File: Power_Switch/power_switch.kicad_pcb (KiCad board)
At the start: 2 copper layers, 22 x 19.2 mm, 6 parts, among them J1 Conn_01x03_Pin, SW1 SW_SPDT

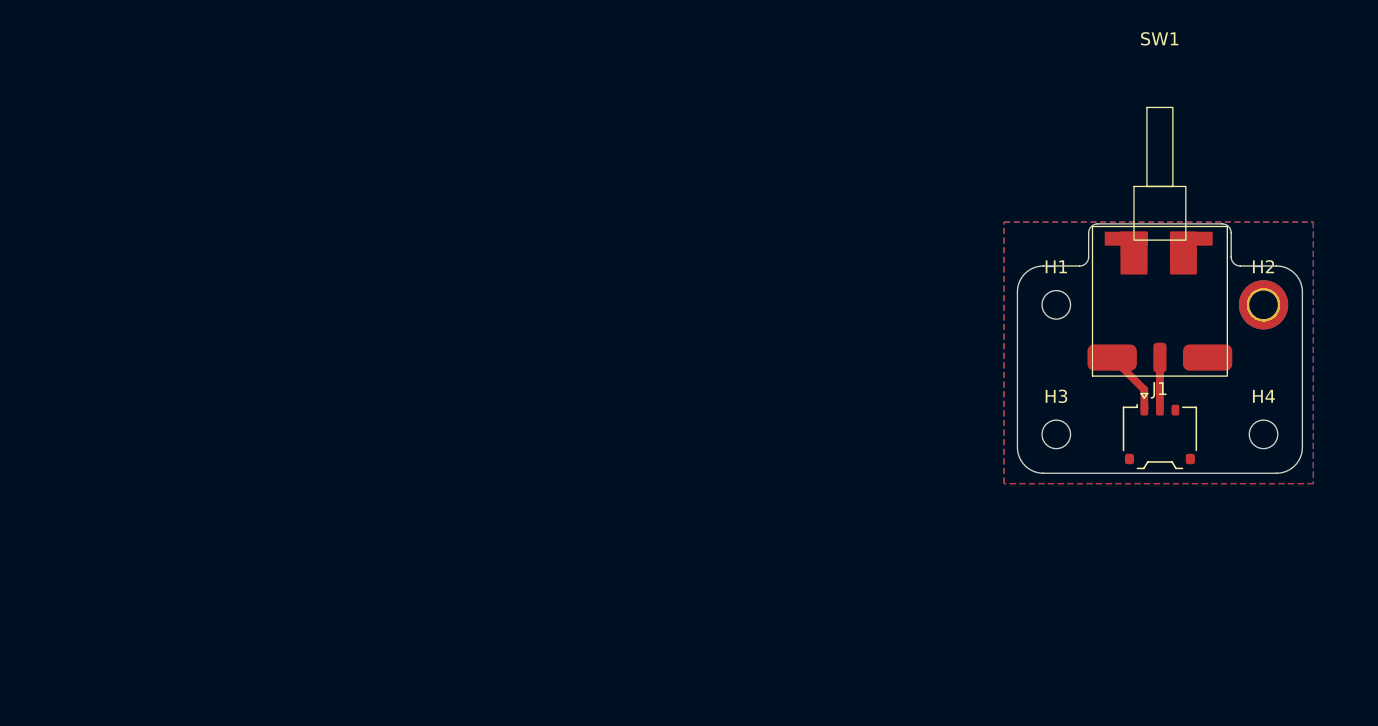
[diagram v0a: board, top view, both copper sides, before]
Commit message: Orginizing and small work done
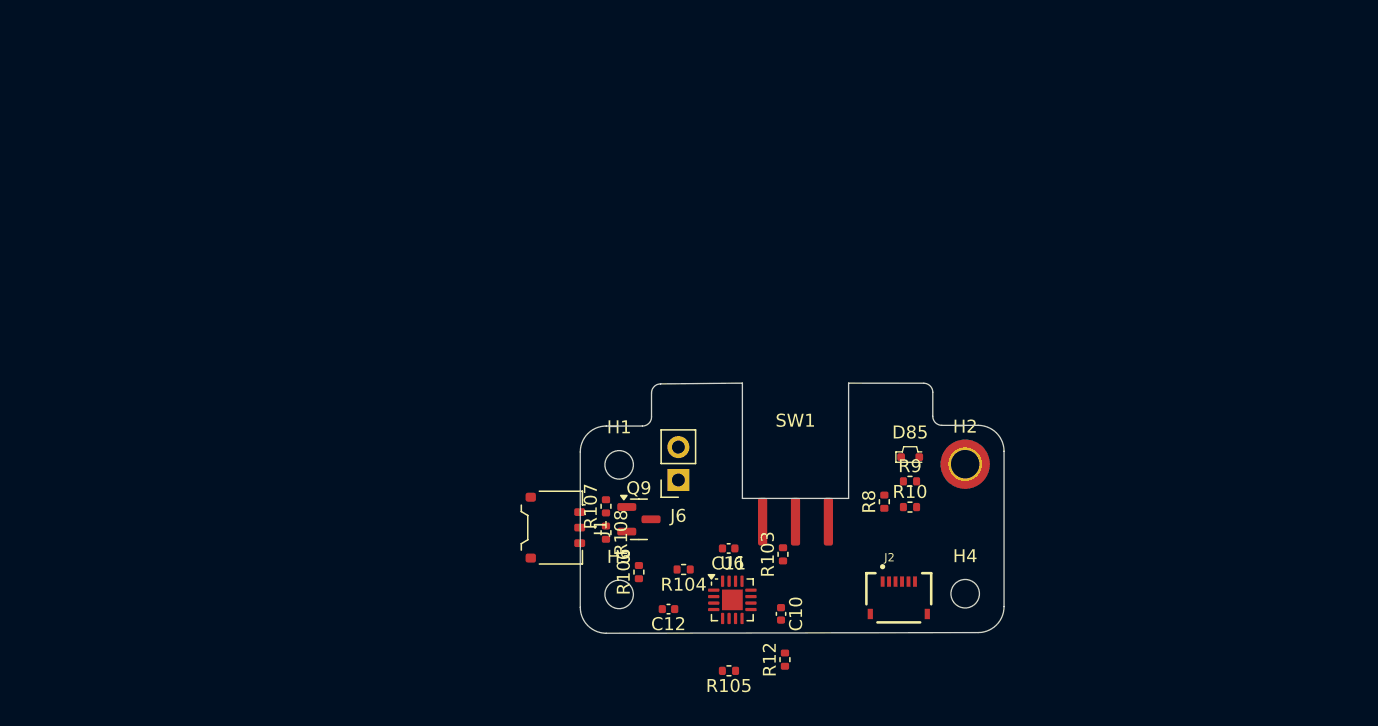
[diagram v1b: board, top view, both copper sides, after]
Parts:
- added C10: 4.7uF, Capacitor_SMD:C_0402_1005Metric, F.Cu at (123.7, 68.9)
- added C11: 1uF, Capacitor_SMD:C_0402_1005Metric, F.Cu at (119.7, 63.8)
- added C12: 1uF, Capacitor_SMD:C_0402_1005Metric, F.Cu at (115.1, 68.5)
- added D85: LED, JohnDeereLibrary:LED_WURTH_155060AS75300, F.Cu at (133.7, 56.8)
- added J2: FFC2B28-06-G, GCT:GCT_FFC2B28-06-G, F.Cu at (132.8, 67.6)
- added J6: Conn_01x02_Pin, Connector_PinSocket_2.54mm:PinSocket_1x02_P2.54mm_Vertical, F.Cu at (115.8, 58.5)
- added Q9: 2N7002, Package_TO_SOT_SMD:SOT-23, F.Cu at (112.8, 61.6)
- added R10: 100k, Resistor_SMD:R_0402_1005Metric, F.Cu at (133.7, 60.6)
- added R103: 1.5k, Resistor_SMD:R_0402_1005Metric, F.Cu at (123.9, 64.3)
- added R104: 3.9k, Resistor_SMD:R_0402_1005Metric, F.Cu at (116.2, 65.4)
- added R105: 47k, Resistor_SMD:R_0402_1005Metric, F.Cu at (119.7, 73.3)
- added R106: 10k, Resistor_SMD:R_0402_1005Metric, F.Cu at (112.8, 65.6)
- added R107: 100R, Resistor_SMD:R_0402_1005Metric, F.Cu at (110.2, 60.6)
- added R108: 10k, Resistor_SMD:R_0402_1005Metric, F.Cu at (110.2, 62.6)
- added R12: 1.5k, Resistor_SMD:R_0402_1005Metric, F.Cu at (124.1, 72.4)
- added R8: 100k, Resistor_SMD:R_0402_1005Metric, F.Cu at (131.7, 60.2)
- added R9: 100k, Resistor_SMD:R_0402_1005Metric, F.Cu at (133.7, 58.6)
- added U6: BQ24075RGT, Package_DFN_QFN:VQFN-16-1EP_3x3mm_P0.5mm_EP1.6x1.6mm, F.Cu at (120.0, 67.8)
- SW1: footprint JohnDeereLibrary:ET01M3D1SAPE -> JohnDeereLibrary:ET01MD1CBE
- moved J1 47.2 mm to (106.3, 62.2), turned to -90 degrees
- moved H1 35.9 mm to (111.3, 57.4)
- moved H3 35.9 mm to (111.3, 67.4)
- moved SW1 33.9 mm to (124.9, 58.9)
- moved H2 26.1 mm to (138.0, 57.3)
- moved H4 26.1 mm to (138.0, 67.3)
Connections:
- J1 pad 1: +BATT -> GND
- J1 pad 2: Net-(J1-Pin_2) -> /TS
- J1 pad 3: GND -> /VBATT
- J1 pad MP: GND -> (no net)
- SW1 pad 1: +BATT -> GND
- SW1 pad 2: Net-(J1-Pin_2) -> SYSOFF
- SW1 pad 3: GND -> Net-(SW1-C)
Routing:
- net +BATT: track 5.08 -> 0.00 mm
- net Net-(J1-Pin_2): track 4.05 -> 0.00 mm
- removed copper zone on B.Cu, net GND
- removed copper zone on F.Cu, net GND
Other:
- board size 22 x 19.2 mm -> 32.7 x 19.3 mm

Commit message: Work done
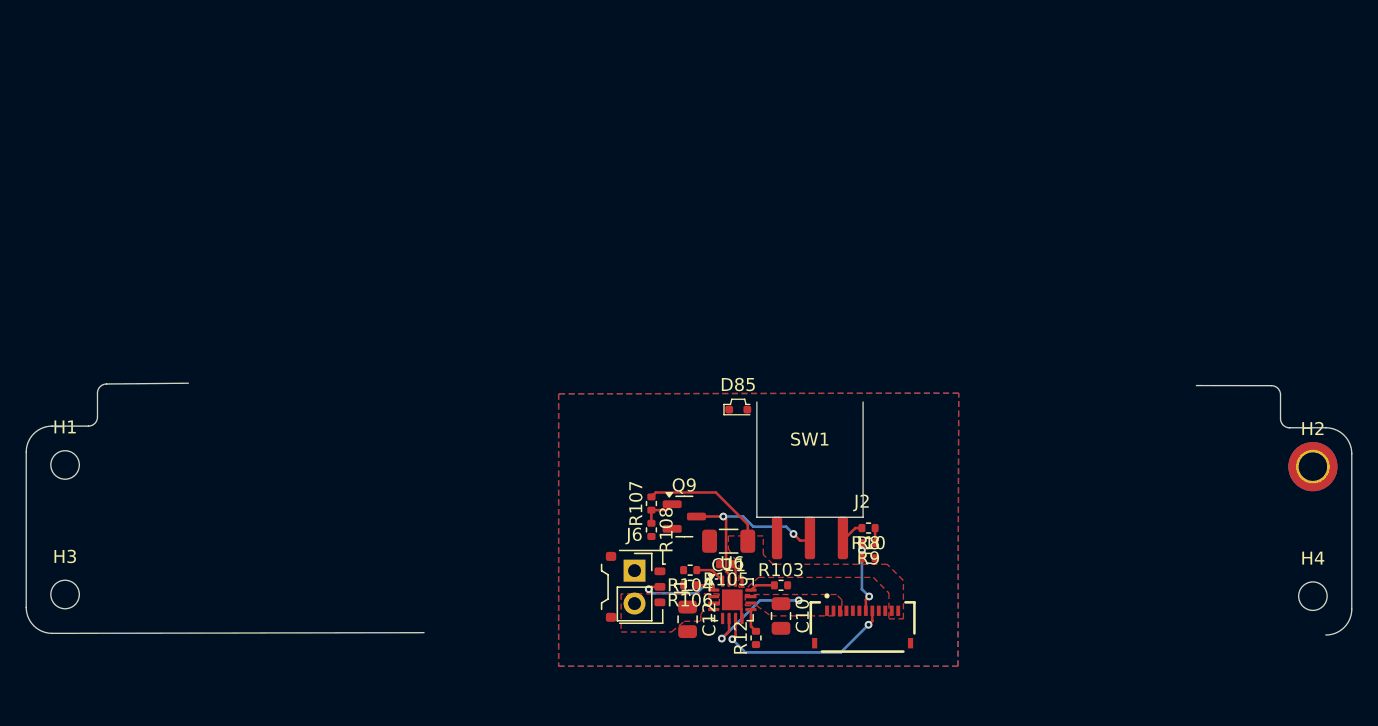
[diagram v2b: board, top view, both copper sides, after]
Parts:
- C10: footprint Capacitor_SMD:C_0402_1005Metric -> Capacitor_SMD:C_0805_2012Metric
- C11: footprint Capacitor_SMD:C_0402_1005Metric -> Capacitor_SMD:C_1206_3216Metric
- C12: value 1uF -> 4.7uF; footprint Capacitor_SMD:C_0402_1005Metric -> Capacitor_SMD:C_0805_2012Metric
- J2: value FFC2B28-06-G -> GCT_FFC2B28-12-G; footprint GCT:GCT_FFC2B28-06-G -> GCT:GCT_FFC2B28-12-G
- R103: value 1.5k -> 1.87k
- R104: value 3.9k -> 1k
- moved H1 42.8 mm to (68.5, 57.4)
- moved H3 42.8 mm to (68.5, 67.4)
- moved H2 26.8 mm to (164.8, 57.5)
- moved H4 26.8 mm to (164.8, 67.5)
- moved D85 13.8 mm to (120.4, 53.1)
- moved R105 8.23 mm to (119.5, 65.0)
- moved J6 7.77 mm to (112.4, 65.5), turned to 0 degrees
- moved J1 7.70 mm to (112.5, 66.8)
- moved R9 5.75 mm to (130.5, 63.4), turned to 180 degrees
- moved R10 5.09 mm to (130.5, 64.6)
- moved R106 4.09 mm to (116.7, 66.6), turned to 180 degrees
- moved Q9 3.51 mm to (116.3, 61.3)
- moved R107 3.51 mm to (113.7, 60.3)
- moved R108 3.51 mm to (113.7, 62.4)
- moved J2 3.16 mm to (130.0, 69.1)
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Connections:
- J2 pad 1: /VDIV -> V_Raw
- J2 pad 2: GND -> V_Raw
- J2 pad 3: /PGOOD -> V_Raw
- J2 pad 4: unconnected-(J2-Pad4) -> GND
- J2 pad 5: VBUS -> GND
- J2 pad 6: V_Raw -> GND
- J2 pad S1: unconnected-(J2-SHIELD-PadS1) -> GND
- J2 pad S2: unconnected-(J2-SHIELD__1-PadS2) -> GND
- R8 pad 1: /VBATT -> VBAT
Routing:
- net /PGOOD: track 0.00 -> 14.7 mm, vias 0 -> 2
- net SYSOFF: track 0.00 -> 14.7 mm, vias 0 -> 2
- net VBUS: track 0.00 -> 9.90 mm
- net V_Raw: track 0.00 -> 8.95 mm, vias 0 -> 2
- net /TS: track 0.00 -> 7.95 mm, vias 0 -> 2
- net /VDIV: track 0.00 -> 6.17 mm, vias 0 -> 2
- net Net-(Q9-G): track 0.00 -> 2.81 mm
- net Net-(U6-ISET): track 0.00 -> 2.36 mm
- net Net-(U6-ILIM): track 0.00 -> 1.97 mm
- net Net-(SW1-C): track 0.00 -> 1.87 mm
- net Net-(U6-~{CHG}): track 0.00 -> 1.84 mm
- net GND: track 0.00 -> 1.75 mm
- net Net-(U6-TMR): track 0.00 -> 1.26 mm
- net VBAT: track 0.00 -> 1.17 mm
- added copper zone on F.Cu, net /VBATT
- added copper zone on B.Cu, net GND
- added copper zone on F.Cu, net GND
- added copper zone on F.Cu, net VBUS
- added copper zone on F.Cu, net V_Raw
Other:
- board size 32.7 x 19.3 mm -> 102.3 x 19.4 mm
